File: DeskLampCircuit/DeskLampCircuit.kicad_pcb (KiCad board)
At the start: 2 copper layers, 40 x 20.1 mm, 20 parts, among them J1 Conn_02x04_Odd_Even, J2 Power in, J3 Conn_01x02_Pin, J5 Conn_01x03_Pin, J6 blueLedConn, J7 redLedConn, J8 greenLedConn, J9 Conn_01x01_Pin, Q1 NPN, Q2 NPN, Q3 NPN, U1 LM317_TO-220

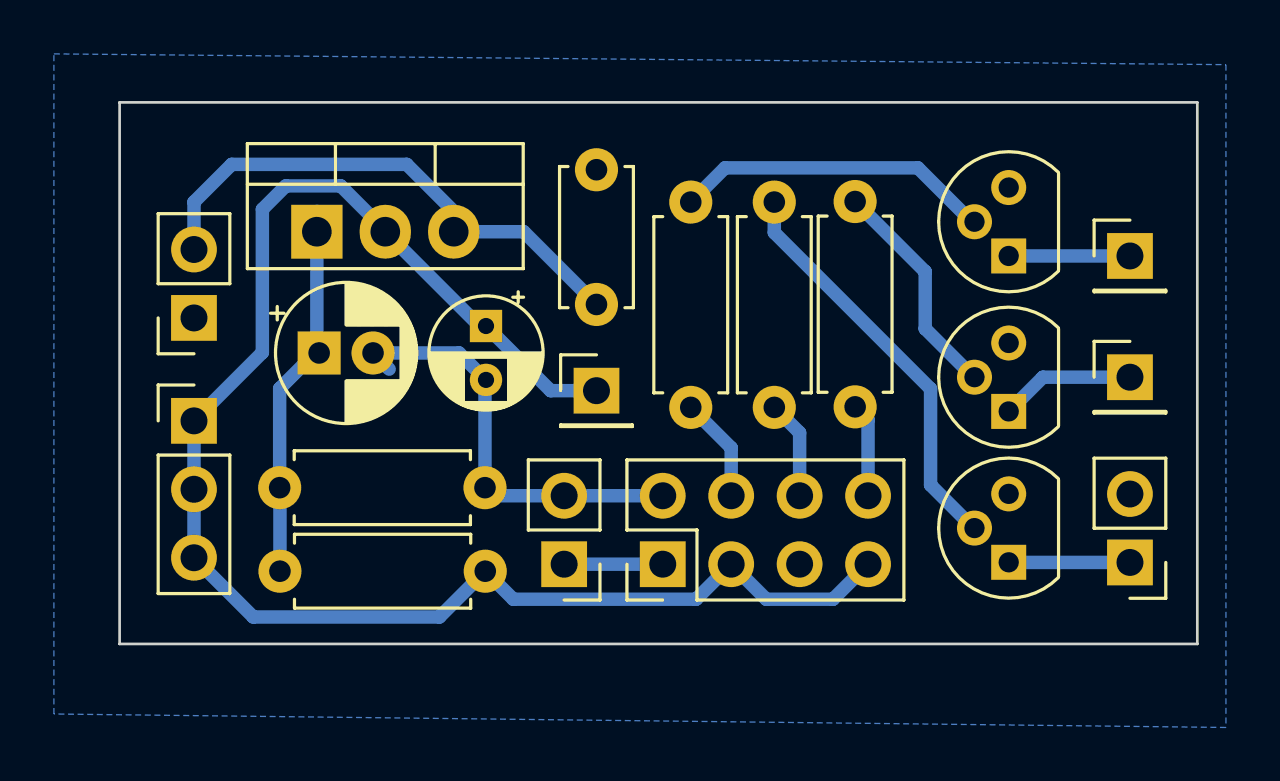
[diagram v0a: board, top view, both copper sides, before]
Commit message: new pcb for leds
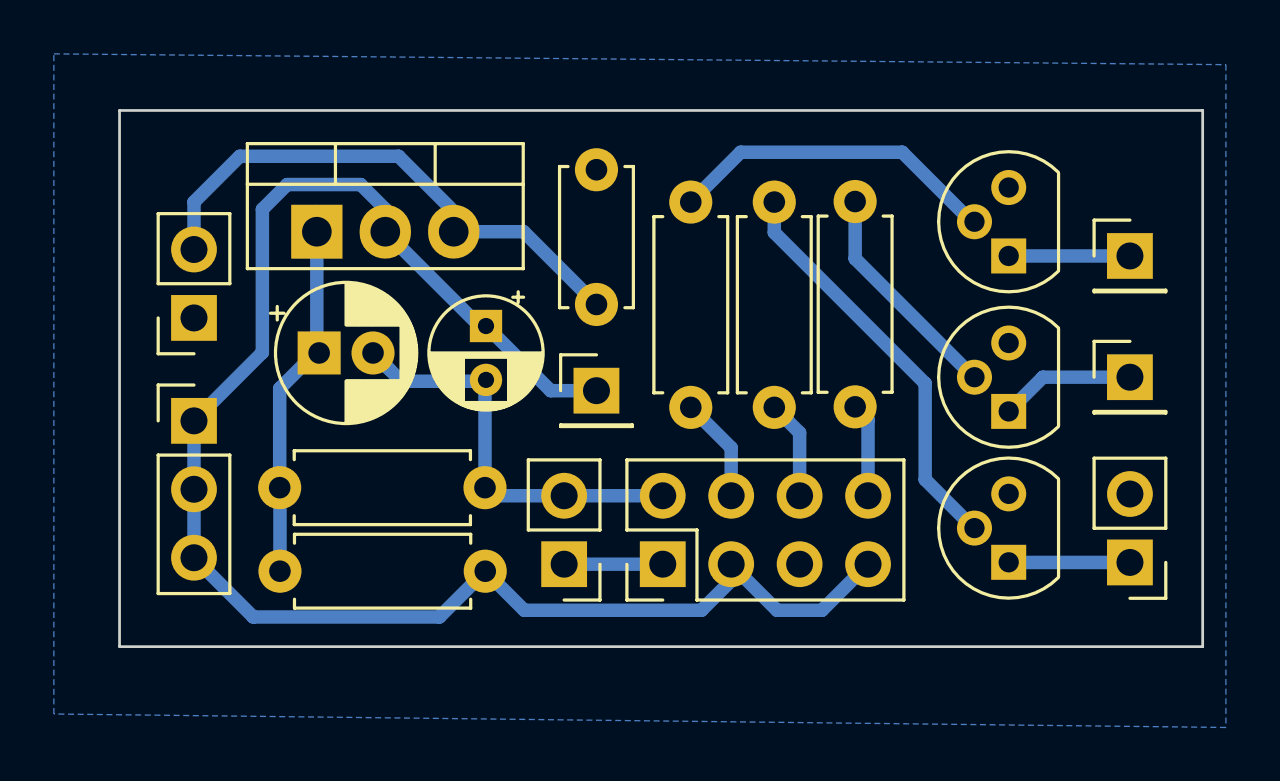
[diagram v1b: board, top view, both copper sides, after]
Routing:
- net +3.3V: track 58.8 -> 60.4 mm
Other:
- board size 40 x 20.1 mm -> 40.2 x 19.9 mm
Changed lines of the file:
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@@
     )
   )
-  (gr_rect (start 20.737818 32.35) (end 60.737818 52.45)
+  (gr_rect (start 20.737818 32.65) (end 60.937818 52.55)
     (stroke (width 0.1) (type default)) (fill none) (layer "Edge.Cuts"))
   (segment (start 28.06 36.395) (end 28.06 41.565112) (width 0.5) (layer "B.Cu") (net 1))
@@
   (segment (start 26.68 46.65) (end 26.68 42.97) (width 0.5) (layer "B.Cu") (net 1))
   (segment (start 34.337818 40.65) (end 34.1 40.65) (width 0.5) (layer "B.Cu") (net 2))
+  (segment (start 36.737818 43.05) (end 34.337818 40.65) (width 0.5) (layer "B.Cu") (net 2))
+  (segment (start 25.7 51.45) (end 23.5 49.25) (width 0.5) (layer "B.Cu") (net 2))
+  (segment (start 29.687818 35.4) (end 26.9575 35.4) (width 0.5) (layer "B.Cu") (net 2))
+  (segment (start 26.037818 41.632182) (end 23.5 44.17) (width 0.5) (layer "B.Cu") (net 2))
+  (segment (start 45.137818 51.2) (end 46.807818 51.2) (width 0.5) (layer "B.Cu") (net 2))
   (segment (start 26.037818 36.319682) (end 26.037818 41.632182) (width 0.5) (layer "B.Cu") (net 2))
-  (segment (start 36.737818 43.05) (end 34.337818 40.65) (width 0.5) (layer "B.Cu") (net 2))
-  (segment (start 26.9075 35.45) (end 26.037818 36.319682) (width 0.5) (layer "B.Cu") (net 2))
-  (segment (start 28.9475 35.45) (end 26.9075 35.45) (width 0.5) (layer "B.Cu") (net 2))
-  (segment (start 43.437818 49.49) (end 44.737818 50.79) (width 0.5) (layer "B.Cu") (net 2))
-  (segment (start 35.35 50.79) (end 42.137818 50.79) (width 0.5) (layer "B.Cu") (net 2))
-  (segment (start 25.7 51.45) (end 23.5 49.25) (width 0.5) (layer "B.Cu") (net 2))
-  (segment (start 44.737818 50.79) (end 47.217818 50.79) (width 0.5) (layer "B.Cu") (net 2))
+  (segment (start 35.76 51.2) (end 42.337818 51.2) (width 0.5) (layer "B.Cu") (net 2))
   (segment (start 23.5 46.71) (end 23.5 44.17) (width 0.5) (layer "B.Cu") (net 2))
-  (segment (start 42.137818 50.79) (end 43.437818 49.49) (width 0.5) (layer "B.Cu") (net 2))
-  (segment (start 26.037818 41.632182) (end 23.5 44.17) (width 0.5) (layer "B.Cu") (net 2))
+  (segment (start 26.9575 35.4) (end 26.037818 36.319682) (width 0.5) (layer "B.Cu") (net 2))
   (segment (start 23.5 49.25) (end 23.5 46.71) (width 0.5) (layer "B.Cu") (net 2))
-  (segment (start 30.6 37.15) (end 30.6 37.1025) (width 0.5) (layer "B.Cu") (net 2))
+  (segment (start 42.337818 51.2) (end 43.437818 50.1) (width 0.5) (layer "B.Cu") (net 2))
   (segment (start 32.61 51.45) (end 25.7 51.45) (width 0.5) (layer "B.Cu") (net 2))
-  (segment (start 34.31 49.75) (end 35.35 50.79) (width 0.5) (layer "B.Cu") (net 2))
+  (segment (start 30.6 37.15) (end 30.6 36.312182) (width 0.5) (layer "B.Cu") (net 2))
+  (segment (start 30.6 36.312182) (end 29.687818 35.4) (width 0.5) (layer "B.Cu") (net 2))
   (segment (start 38.437818 43.05) (end 36.737818 43.05) (width 0.5) (layer "B.Cu") (net 2))
-  (segment (start 30.6 37.1025) (end 28.9475 35.45) (width 0.5) (layer "B.Cu") (net 2))
+  (segment (start 43.437818 49.5) (end 45.137818 51.2) (width 0.5) (layer "B.Cu") (net 2))
+  (segment (start 46.807818 51.2) (end 48.517818 49.49) (width 0.5) (layer "B.Cu") (net 2))
   (segment (start 34.31 49.75) (end 32.61 51.45) (width 0.5) (layer "B.Cu") (net 2))
+  (segment (start 34.31 49.75) (end 35.76 51.2) (width 0.5) (layer "B.Cu") (net 2))
+  (segment (start 43.437818 49.49) (end 43.437818 49.5) (width 0.5) (layer "B.Cu") (net 2))
+  (segment (start 43.437818 50.1) (end 43.437818 49.49) (width 0.5) (layer "B.Cu") (net 2))
   (segment (start 30.6 37.15) (end 30.837818 37.15) (width 0.5) (layer "B.Cu") (net 2))
   (segment (start 34.1 40.65) (end 30.6 37.15) (width 0.5) (layer "B.Cu") (net 2))
-  (segment (start 47.217818 50.79) (end 48.517818 49.49) (width 0.5) (layer "B.Cu") (net 2))
+  (segment (start 48.517818 46.95) (end 48.517818 44.13) (width 0.5) (layer "B.Cu") (net 3))
   (segment (start 48.517818 44.13) (end 48.037818 43.65) (width 0.5) (layer "B.Cu") (net 3))
-  (segment (start 48.517818 46.95) (end 48.517818 44.13) (width 0.5) (layer "B.Cu") (net 3))
   (segment (start 45.977818 44.61) (end 45.037818 43.67) (width 0.5) (layer "B.Cu") (net 4))
   (segment (start 45.977818 46.95) (end 45.977818 44.61) (width 0.5) (layer "B.Cu") (net 4))
   (segment (start 40.897818 49.49) (end 37.237818 49.49) (width 0.5) (layer "B.Cu") (net 5))
   (segment (start 37.237818 46.95) (end 34.6 46.95) (width 0.5) (layer "B.Cu") (net 6))
+  (segment (start 34.337818 42.65) (end 34.287818 42.7) (width 0.5) (layer "B.Cu") (net 6))
   (segment (start 34.6 46.95) (end 34.3 46.65) (width 0.5) (layer "B.Cu") (net 6))
   (segment (start 37.237818 46.95) (end 40.897818 46.95) (width 0.5) (layer "B.Cu") (net 6))
   (segment (start 34.3 42.8774) (end 34.3 46.65) (width 0.5) (layer "B.Cu") (net 6))
-  (segment (start 34.337818 42.65) (end 33.337818 41.65) (width 0.5) (layer "B.Cu") (net 6))
+  (segment (start 34.287818 42.7) (end 31.194888 42.7) (width 0.5) (layer "B.Cu") (net 6))
   (segment (start 30.744888 42.25) (end 30.144888 41.65) (width 0.5) (layer "B.Cu") (net 6))
-  (segment (start 33.337818 41.65) (end 30.144888 41.65) (width 0.5) (layer "B.Cu") (net 6))
+  (segment (start 31.194888 42.7) (end 30.144888 41.65) (width 0.5) (layer "B.Cu") (net 6))
   (segment (start 43.437818 46.95) (end 43.437818 45.17) (width 0.5) (layer "B.Cu") (net 7))
   (segment (start 43.437818 45.17) (end 41.937818 43.67) (width 0.5) (layer "B.Cu") (net 7))
+  (segment (start 31.095 34.35) (end 33.14 36.395) (width 0.5) (layer "B.Cu") (net 8))
+  (segment (start 25.2 34.35) (end 31.095 34.35) (width 0.5) (layer "B.Cu") (net 8))
+  (segment (start 35.737818 37.15) (end 38.437818 39.85) (width 0.5) (layer "B.Cu") (net 8))
   (segment (start 23.5 37.81) (end 23.5 36.05) (width 0.5) (layer "B.Cu") (net 8))
-  (segment (start 24.9 34.65) (end 31.395 34.65) (width 0.5) (layer "B.Cu") (net 8))
-  (segment (start 35.737818 37.15) (end 38.437818 39.85) (width 0.5) (layer "B.Cu") (net 8))
-  (segment (start 23.5 36.05) (end 24.9 34.65) (width 0.5) (layer "B.Cu") (net 8))
+  (segment (start 23.5 36.05) (end 25.2 34.35) (width 0.5) (layer "B.Cu") (net 8))
+  (segment (start 33.14 37.15) (end 35.737818 37.15) (width 0.5) (layer "B.Cu") (net 8))
   (segment (start 33.14 36.395) (end 33.14 37.15) (width 0.5) (layer "B.Cu") (net 8))
-  (segment (start 33.14 37.15) (end 35.737818 37.15) (width 0.5) (layer "B.Cu") (net 8))
-  (segment (start 31.395 34.65) (end 33.14 36.395) (width 0.5) (layer "B.Cu") (net 8))
-  (segment (start 50.637818 40.75) (end 50.637818 38.63) (width 0.5) (layer "B.Cu") (net 10))
-  (segment (start 50.637818 38.63) (end 48.037818 36.03) (width 0.5) (layer "B.Cu") (net 10))
-  (segment (start 52.437818 42.55) (end 50.637818 40.75) (width 0.5) (layer "B.Cu") (net 10))
-  (segment (start 50.837818 42.98137) (end 50.837818 46.55) (width 0.5) (layer "B.Cu") (net 11))
-  (segment (start 45.037818 37.18137) (end 50.837818 42.98137) (width 0.5) (layer "B.Cu") (net 11))
+  (segment (start 52.437818 42.55) (end 48.037818 38.15) (width 0.5) (layer "B.Cu") (net 10))
+  (segment (start 48.037818 38.15) (end 48.037818 36.03) (width 0.5) (layer "B.Cu") (net 10))
+  (segment (start 52.437818 48.15) (end 52.537818 48.15) (width 0.5) (layer "B.Cu") (net 11))
+  (segment (start 50.637818 42.78137) (end 50.637818 46.35) (width 0.5) (layer "B.Cu") (net 11))
   (segment (start 45.037818 36.05) (end 45.037818 37.18137) (width 0.5) (layer "B.Cu") (net 11))
-  (segment (start 50.837818 46.55) (end 52.437818 48.15) (width 0.5) (layer "B.Cu") (net 11))
-  (segment (start 52.437818 48.15) (end 52.537818 48.15) (width 0.5) (layer "B.Cu") (net 11))
-  (segment (start 52.367818 36.78) (end 50.367818 34.78) (width 0.5) (layer "B.Cu") (net 12))
-  (segment (start 50.367818 34.78) (end 43.207818 34.78) (width 0.5) (layer "B.Cu") (net 12))
-  (segment (start 43.207818 34.78) (end 41.937818 36.05) (width 0.5) (layer "B.Cu") (net 12))
+  (segment (start 50.637818 46.35) (end 52.437818 48.15) (width 0.5) (layer "B.Cu") (net 11))
+  (segment (start 45.037818 37.18137) (end 50.637818 42.78137) (width 0.5) (layer "B.Cu") (net 11))
+  (segment (start 52.367818 36.78) (end 49.787818 34.2) (width 0.5) (layer "B.Cu") (net 12))
+  (segment (start 43.787818 34.2) (end 41.937818 36.05) (width 0.5) (layer "B.Cu") (net 12))
+  (segment (start 49.787818 34.2) (end 43.787818 34.2) (width 0.5) (layer "B.Cu") (net 12))
   (segment (start 53.737818 38.05) (end 58.237818 38.05) (width 0.5) (layer "B.Cu") (net 13))
   (segment (start 55.007818 42.55) (end 53.737818 43.82) (width 0.5) (layer "B.Cu") (net 14))
